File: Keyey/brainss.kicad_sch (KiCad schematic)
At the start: 37 parts, among them J1 USB_C_Receptacle_USB2.0_16P, SW3 SW_Push, SW7 SW_Push, U2 RP2350B, U3 NCP1117-3.3_SOT223, U4 W25Q128JVS, Y1 ABM8-272-T3

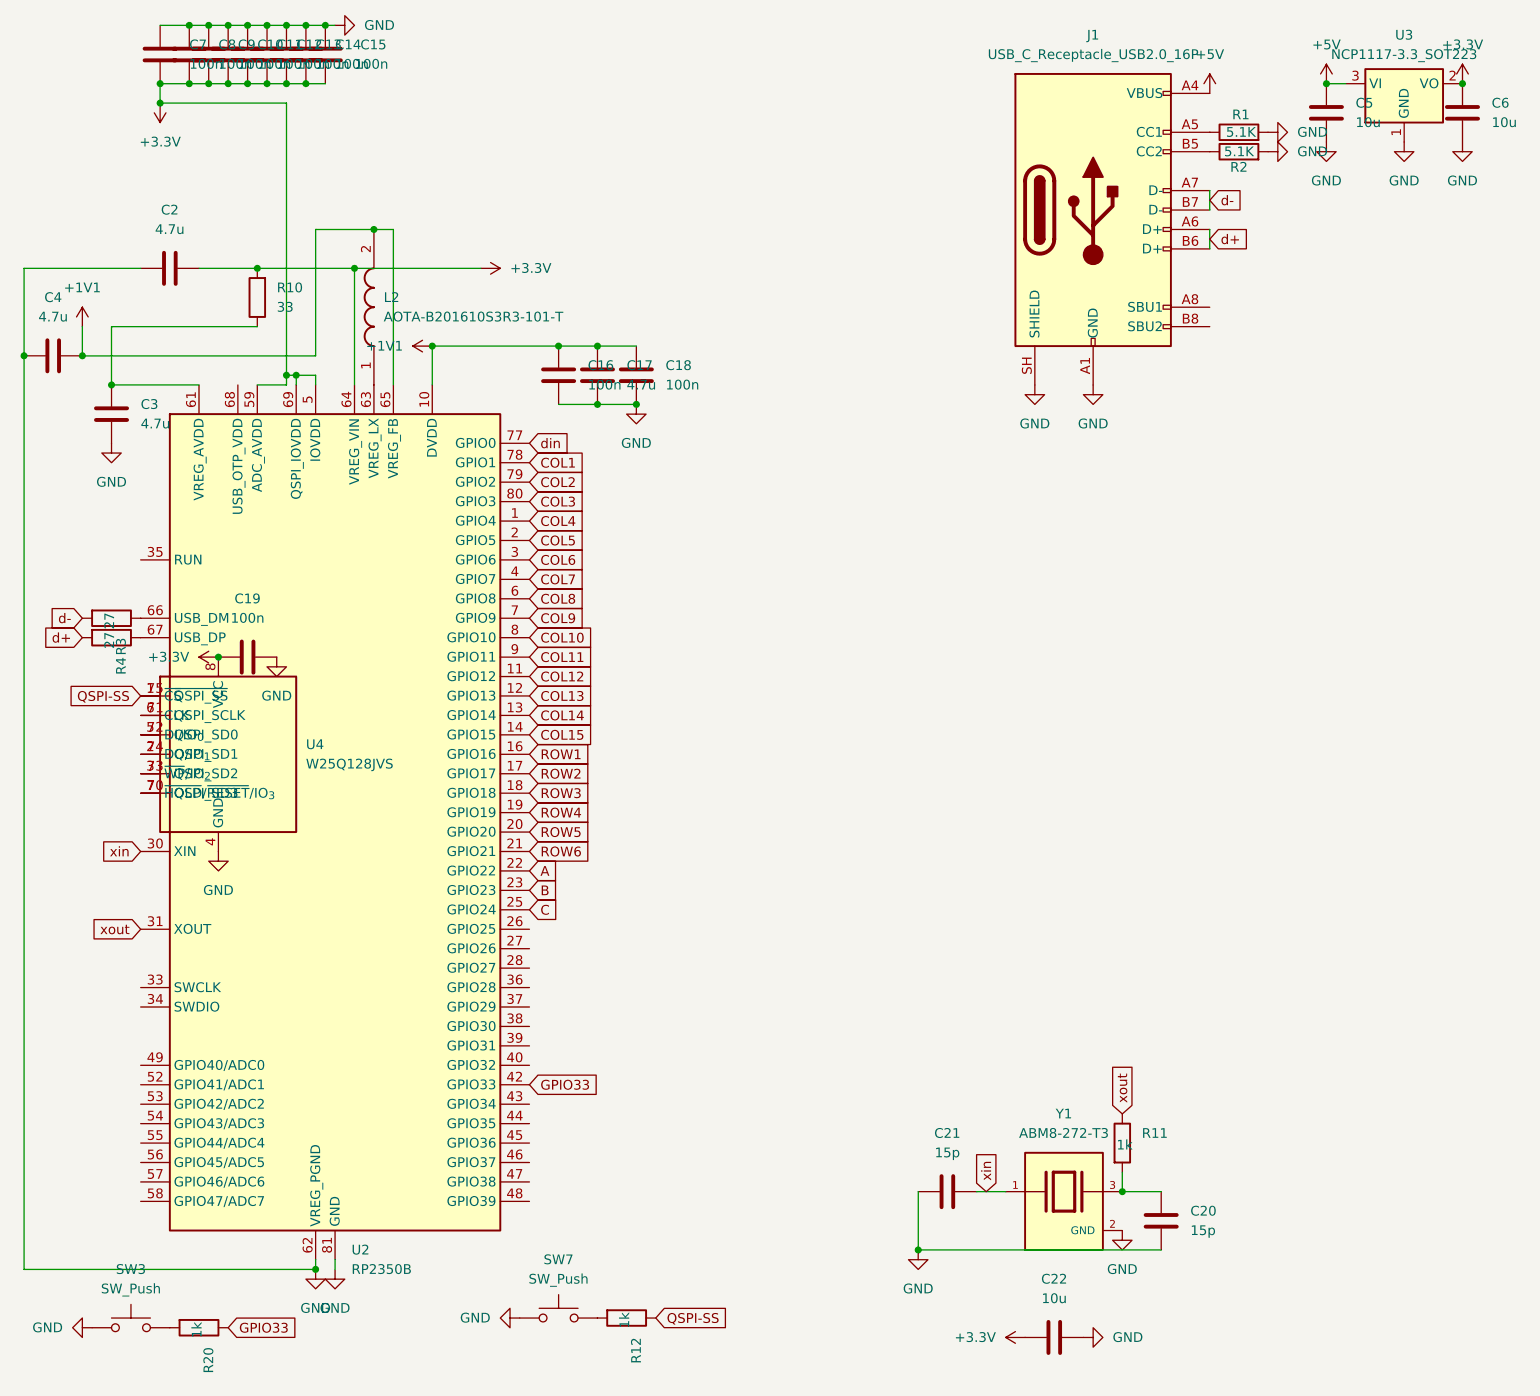
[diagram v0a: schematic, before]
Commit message: keyey
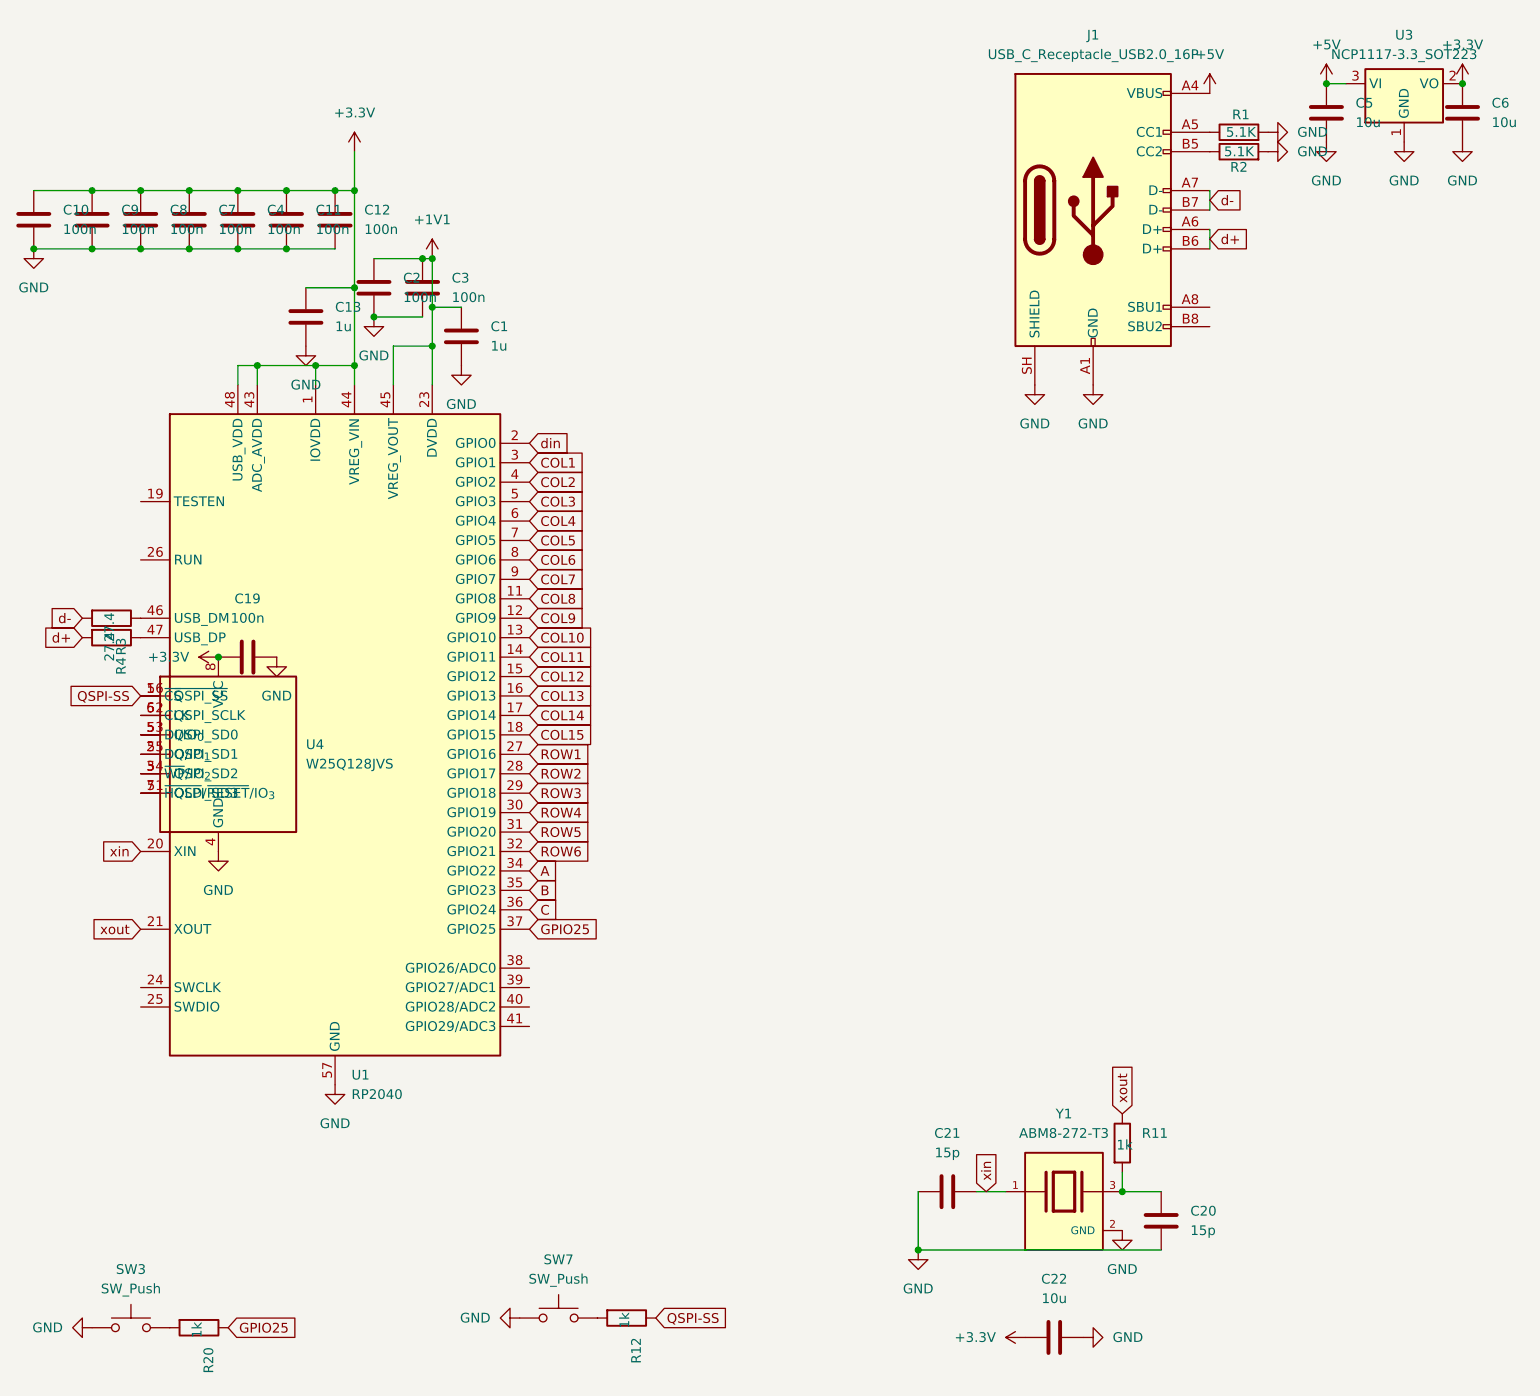
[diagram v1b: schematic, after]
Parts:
- removed C14, C15, C16, C18: 100n, Capacitor_SMD:C_0402_1005Metric_Pad0.74x0.62mm_HandSolder, symbol Device:C
- removed C17: 4.7u, Capacitor_SMD:C_0402_1005Metric_Pad0.74x0.62mm_HandSolder, symbol Device:C
- removed L2: AOTA-B201610S3R3-101-T, AOTA-B201610S3R3-101-T:AOTAB201610S3R3101T, symbol AOTA-B201610S3R3-101-T:AOTA-B201610S3R3-101-T
- removed R10: 33, Resistor_SMD:R_0402_1005Metric_Pad0.72x0.64mm_HandSolder, symbol Device:R
- removed U2: RP2350B, Package_DFN_QFN:QFN-80-1EP_10x10mm_P0.4mm_EP3.4x3.4mm, symbol MCU_RaspberryPi:RP2350B
- added C1: 1u, Capacitor_SMD:C_0402_1005Metric, symbol Device:C
- added U1: RP2040, Package_DFN_QFN:QFN-56-1EP_7x7mm_P0.4mm_EP3.2x3.2mm, symbol MCU_RaspberryPi:RP2040
- C10, C11, C12, C7, C8, C9: footprint Capacitor_SMD:C_0402_1005Metric_Pad0.74x0.62mm_HandSolder -> Capacitor_SMD:C_0402_1005Metric
- C13: value 100n -> 1u; footprint Capacitor_SMD:C_0402_1005Metric_Pad0.74x0.62mm_HandSolder -> Capacitor_SMD:C_0402_1005Metric
- C2, C3, C4: value 4.7u -> 100n; footprint Capacitor_SMD:C_0402_1005Metric_Pad0.74x0.62mm_HandSolder -> Capacitor_SMD:C_0402_1005Metric
- C5, C6: footprint Capacitor_SMD:C_01005_0402Metric_Pad0.57x0.30mm_HandSolder -> Capacitor_SMD:C_0402_1005Metric_Pad0.74x0.62mm_HandSolder
- R3, R4: value 27 -> 27.4
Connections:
- net +1V1: now also C2.1, C3.1, C1.1, U1.23 (DVDD), U1.45 (VREG_VOUT), U1.50 (DVDD); no longer C4.2
- net +3.3V: now also C4.1, U1.1 (IOVDD), U1.10 (IOVDD), U1.22 (IOVDD), U1.33 (IOVDD), U1.42 (IOVDD), U1.43 (ADC_AVDD), U1.44 (VREG_VIN), U1.48 (USB_VDD), U1.49 (IOVDD); no longer C2.2
- net A: now also U1.34 (GPIO22)
- net B: now also U1.35 (GPIO23)
- net C: now also U1.36 (GPIO24)
- net COL1: now also U1.3 (GPIO1)
- net COL10: now also U1.13 (GPIO10)
- net COL11: now also U1.14 (GPIO11)
- net COL12: now also U1.15 (GPIO12)
- net COL13: now also U1.16 (GPIO13)
- net COL14: now also U1.17 (GPIO14)
- net COL15: now also U1.18 (GPIO15)
- net COL2: now also U1.4 (GPIO2)
- net COL3: now also U1.5 (GPIO3)
- net COL4: now also U1.6 (GPIO4)
- net COL5: now also U1.7 (GPIO5)
- net COL6: now also U1.8 (GPIO6)
- net COL7: now also U1.9 (GPIO7)
- net COL8: now also U1.11 (GPIO8)
- net COL9: now also U1.12 (GPIO9)
- net GND: now also C2.2, C3.2, C4.2, C1.2, U1.57 (GND); no longer C2.1, C3.1, C4.1
- net QSPI-SS: now also U1.56 (~{QSPI_SS})
- net ROW1: now also U1.27 (GPIO16)
- net ROW2: now also U1.28 (GPIO17)
- net ROW3: now also U1.29 (GPIO18)
- net ROW4: now also U1.30 (GPIO19)
- net ROW5: now also U1.31 (GPIO20)
- net ROW6: now also U1.32 (GPIO21)
- net din: now also U1.2 (GPIO0)
- net xin: now also U1.20 (XIN)
- net xout: now also U1.21 (XOUT)
- net at R3.1: now also U1.46 (USB_DM)
- net at U4.2 (DO/IO_{1}): now also U1.55 (QSPI_SD1)
- net at U4.3 (~{WP}/IO_{2}): now also U1.54 (QSPI_SD2)
- net at U4.5 (DI/IO_{0}): now also U1.53 (QSPI_SD0)
- net at U4.6 (CLK): now also U1.52 (QSPI_SCLK)
- net at U4.7 (~{HOLD}/~{RESET}/IO_{3}): now also U1.51 (QSPI_SD3)
- net at R4.1: now also U1.47 (USB_DP)
- net GPIO33 renamed GPIO25
- net GPIO25: now also U1.37 (GPIO25)
